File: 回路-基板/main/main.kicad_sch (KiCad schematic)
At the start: 45 parts, among them J2 Conn_01x06_Pin, Q1 PNP, Q2 NPN, Q3 PNP, Q4 NPN, SW1 SW_Push, SW2 SW_Push, SW3 SW_Push, SW4 SW_Push, SW5 SW_Push, SW6 SW_SPDT, U1 TWE-L-WX, U3 LM1117MP-3.3

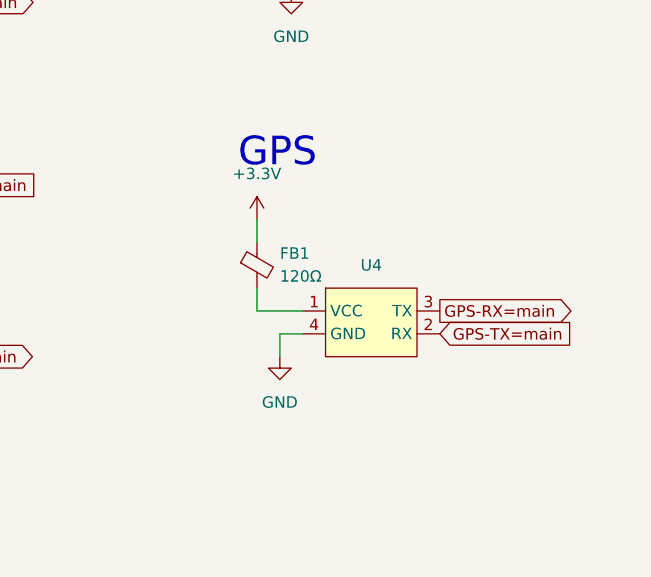
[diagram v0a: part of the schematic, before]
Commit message: 回路関連
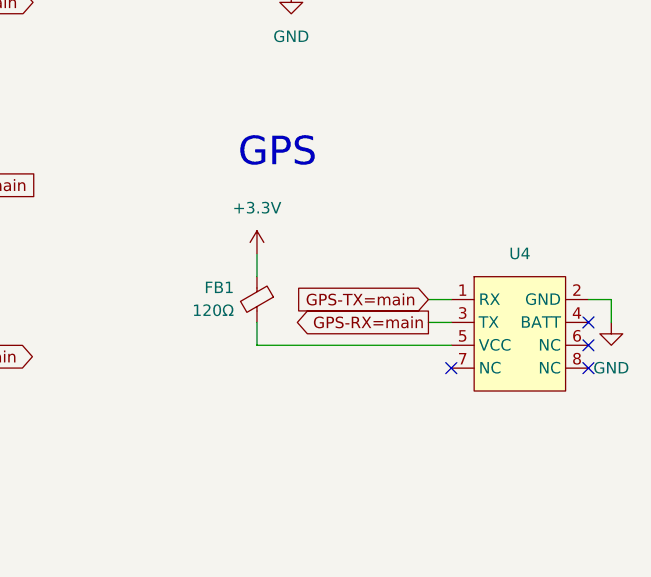
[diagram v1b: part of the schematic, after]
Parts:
- removed U4: ~, @2024-cansat:GPS-54D-014, symbol CanSat:GY-NEO6MV2
- added U4: ~, @2024-cansat:GPS-54D-014, symbol @cansat:GPS-54DB-014
- C10, C6, C7, C8, C9: footprint (none) -> Capacitor_SMD:C_0805_2012Metric
- FB1: footprint (none) -> Inductor_SMD:L_0603_1608Metric
- JP1, JP3: footprint (none) -> Jumper:SolderJumper-2_P1.3mm_Bridged_Pad1.0x1.5mm
- JP2, JP4: footprint (none) -> Jumper:SolderJumper-2_P1.3mm_Open_Pad1.0x1.5mm
- R10, R11, R12, R13: footprint (none) -> Resistor_SMD:R_0805_2012Metric
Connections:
- net GND: now also U4.2 (GND)
- net GPS-RX=main: now also U4.3 (TX)
- net GPS-TX=main: now also U4.1 (RX)
- net at FB1.2: now also U4.5 (VCC)
- no-connect marks 12 -> 16
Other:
- moved on the sheet: FB1
